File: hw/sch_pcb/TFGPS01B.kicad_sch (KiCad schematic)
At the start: 74 parts, among them J1 SM10B-GHS-TB, J2 USBC_USB4105-GF-A, J3 SM06B-GHS-TB, J4 SM04B-GHS-TB, J5 SM08B-GHS-TB, M1 HOLE, M2 HOLE, M3 HOLE, M4 HOLE, Q1 BC817-25, Q2 BC817-25, Q3 BC817-25, U1 MIC5504-3.3YM5, U2 USBLC6-2SC6, U3 NEO-M8P, U4 MAX2655

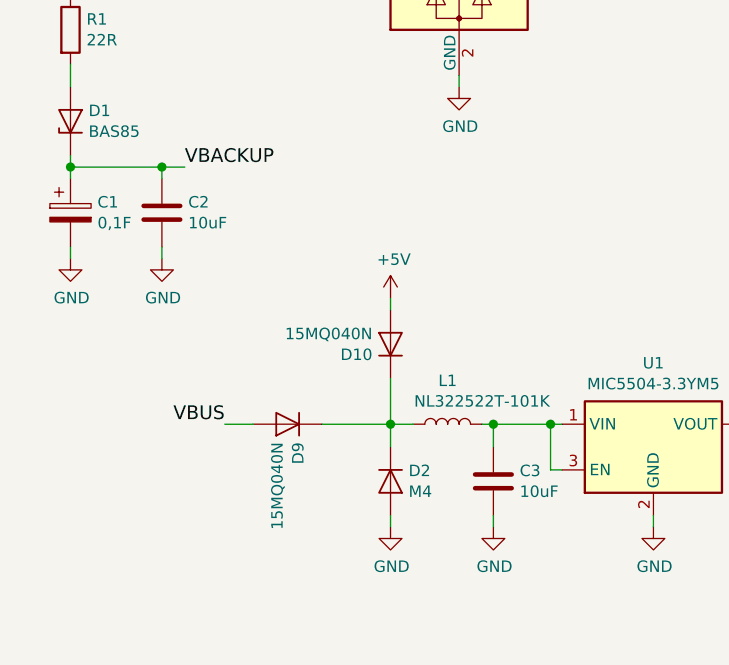
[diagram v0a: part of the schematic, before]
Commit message: Edit SCH
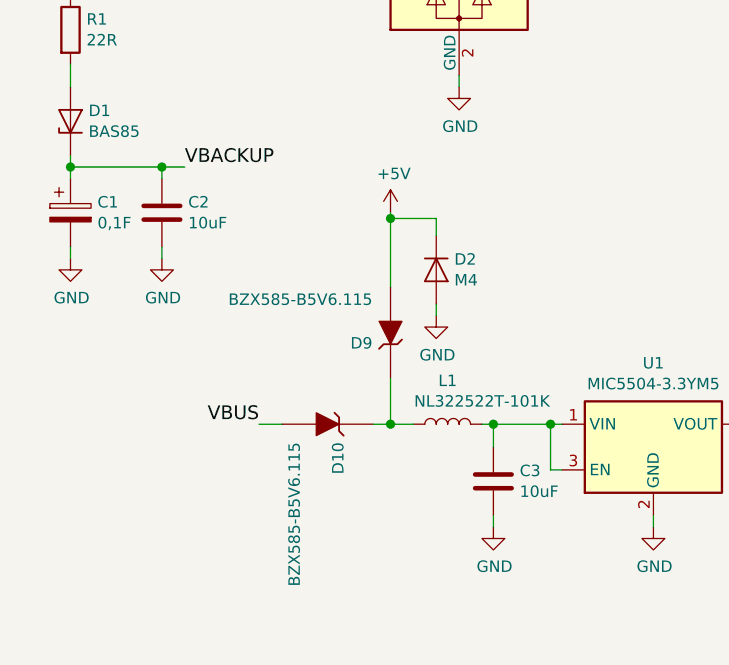
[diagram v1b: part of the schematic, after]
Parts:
- removed D10, D9: 15MQ040N, Diode_SMD:D_SMA, symbol Device:D
- added D10, D9: BZX585-B5V6.115, Diode_SMD:D_SOD-523, symbol MLAB_D:D_ZENER
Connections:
- net +5V: now also D2.1 (K), D9.2 (A)
- net VBUS: now also D10.2 (A)
- net at L1.1: now also D10.1 (K), D9.1 (K); no longer D2.1 (K)
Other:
- moved on the sheet: D2

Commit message: Edit PCB
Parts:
- C13: UST_ID (none) -> 60d587411287500165f85b5f
- L2: UST_ID (none) -> 5c70984412875079b91f8803
- R13, R25: UST_ID (none) -> 5c70984612875079b91f899f
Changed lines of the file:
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@@
       (effects (font (size 1.27 1.27)) hide)
     )
-    (property "UST_ID" "" (id 4) (at 250.19 99.06 0)
+    (property "UST_ID" "5c70984412875079b91f8803" (id 4) (at 250.19 99.06 0)
       (effects (font (size 1.27 1.27)) hide)
     )
@@
       (effects (font (size 1.27 1.27)) hide)
     )
-    (property "UST_ID" "" (id 4) (at 144.78 180.34 0)
+    (property "UST_ID" "5c70984612875079b91f899f" (id 4) (at 144.78 180.34 0)
       (effects (font (size 1.27 1.27)) hide)
     )
@@
       (effects (font (size 1.27 1.27)) hide)
     )
-    (property "UST_ID" "" (id 4) (at 152.4 37.465 0)
+    (property "UST_ID" "5c70984612875079b91f899f" (id 4) (at 152.4 37.465 0)
       (effects (font (size 1.27 1.27)) hide)
     )
@@
       (effects (font (size 1.27 1.27)) hide)
     )
-    (property "UST_ID" "" (id 4) (at 256.54 105.41 0)
-      (effects (font (size 1.27 1.27)) hide)
-    )
+    (property "UST_ID" "60d587411287500165f85b5f" (id 4) (at 256.54 105.41 0)
+      (effects (font (size 1.27 1.27)) hide)
+    )

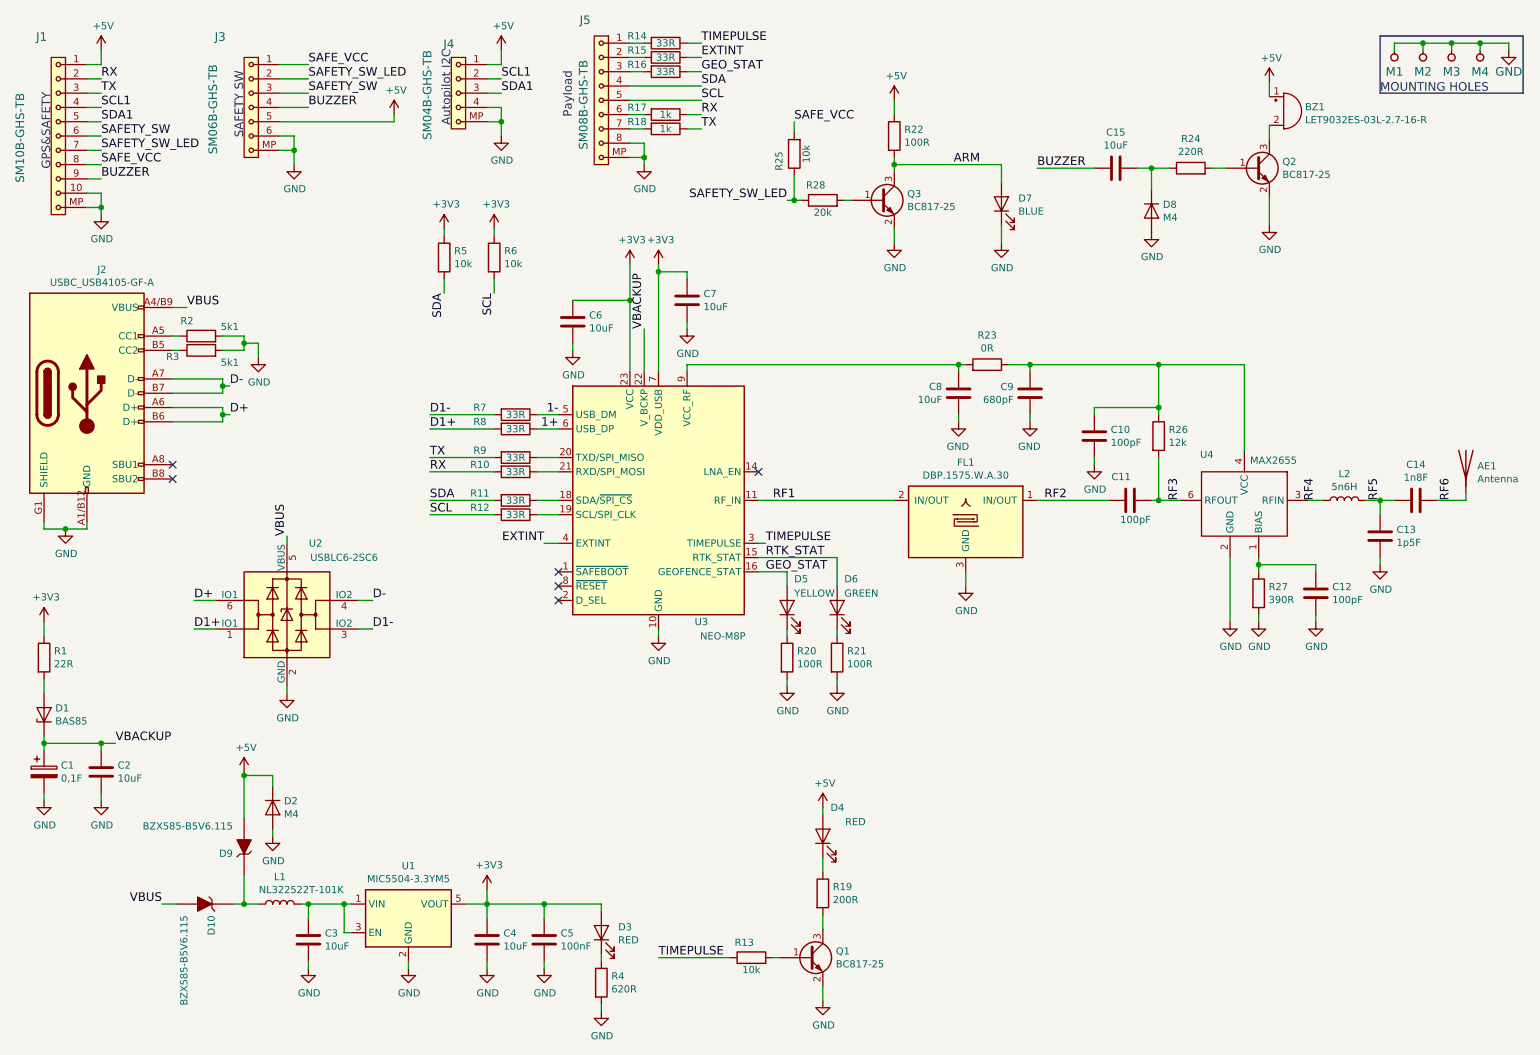
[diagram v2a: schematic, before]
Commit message: Uprava projektovych dat
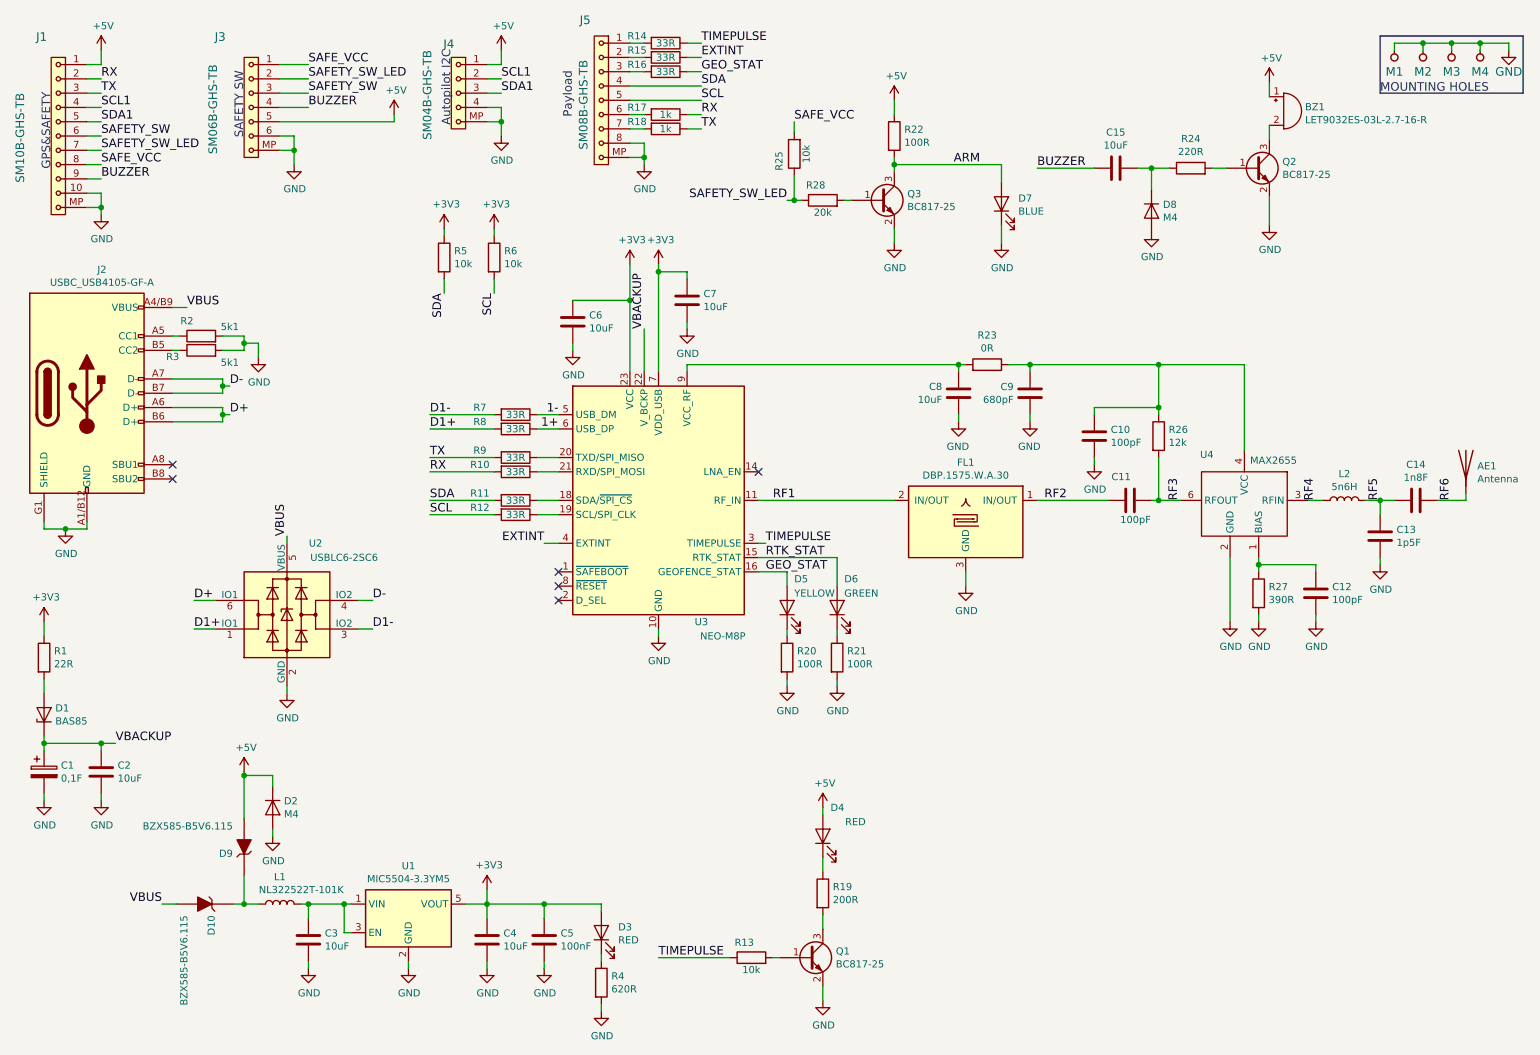
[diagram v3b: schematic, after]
